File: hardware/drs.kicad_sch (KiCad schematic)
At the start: 0 parts

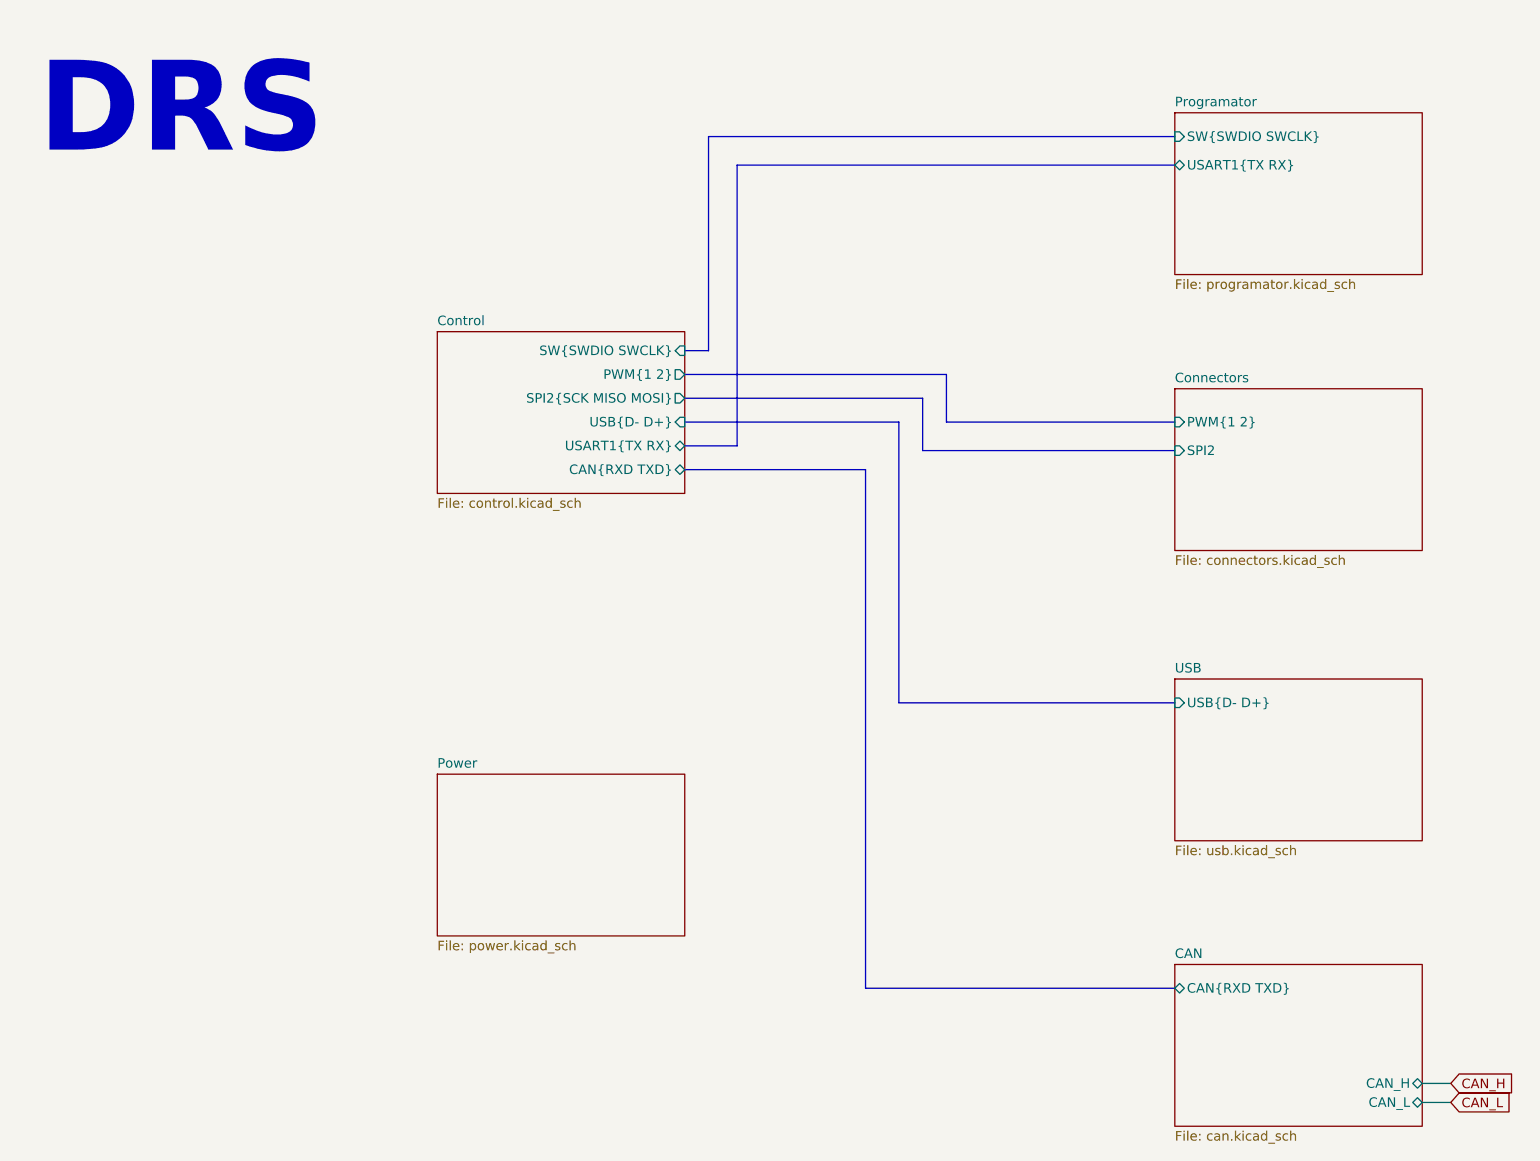
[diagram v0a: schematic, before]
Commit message: Poprawione busy, brak errorow
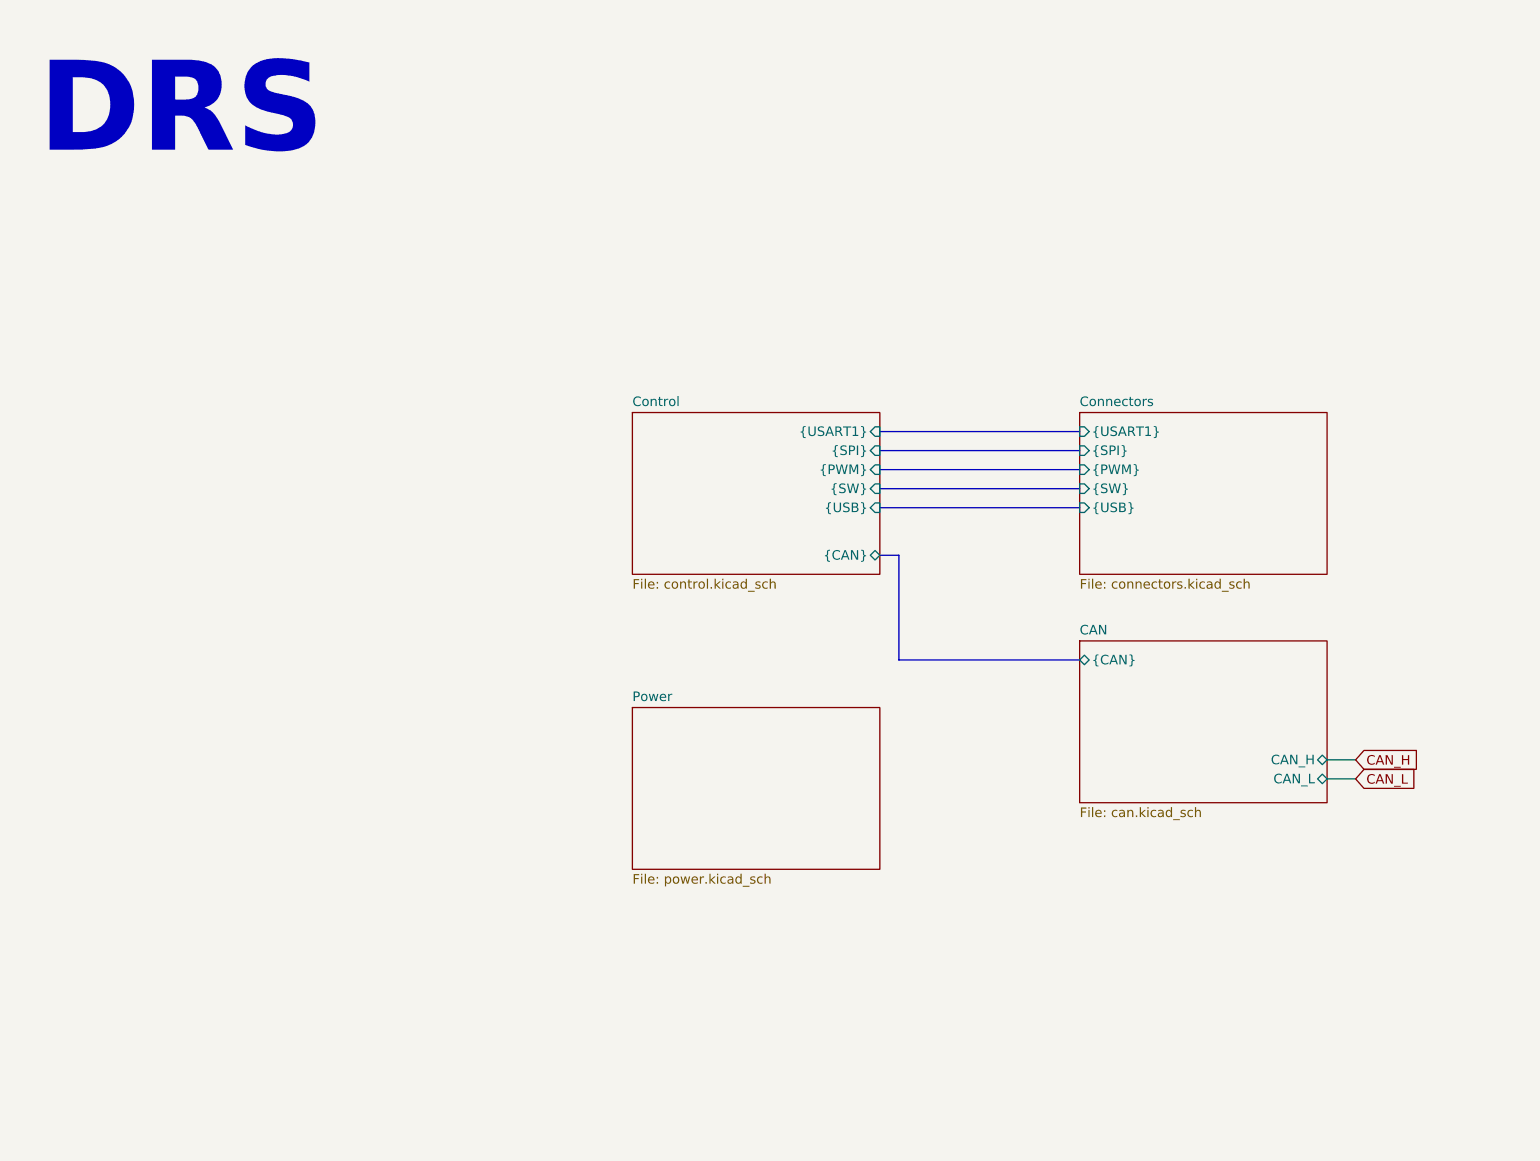
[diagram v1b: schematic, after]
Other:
- removed sheet Programator
- removed sheet USB
- sheet CAN ports: added {CAN}; removed CAN{RXD TXD}
- sheet Connectors ports: added {PWM}, {SPI}, {SW}, {USART1}, {USB}; removed PWM{1 2}, SPI2
- sheet Control ports: added {CAN}, {PWM}, {SPI}, {SW}, {USART1}, {USB}; removed CAN{RXD TXD}, PWM{1 2}, SPI2{SCK MISO MOSI}, SW{SWDIO SWCLK}, USART1{TX RX}, USB{D- D+}
